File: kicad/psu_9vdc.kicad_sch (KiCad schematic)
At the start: 5 parts, among them U1 LM7809_TO220

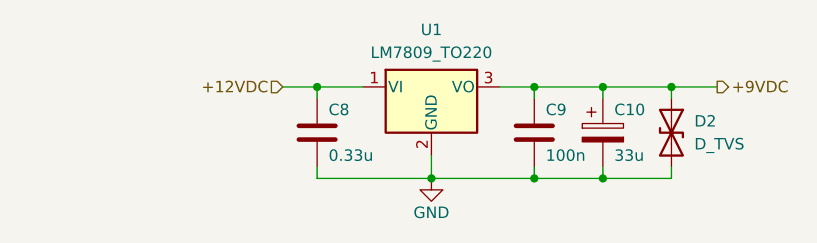
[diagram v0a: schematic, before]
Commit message: Post zip cleanups
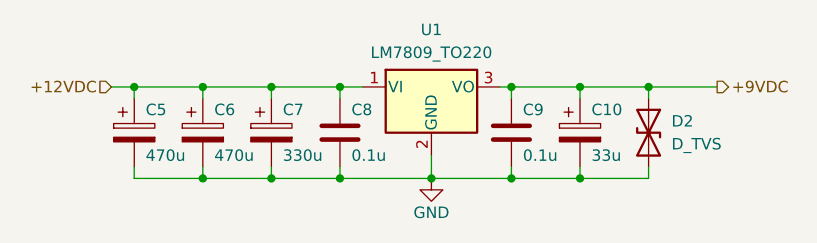
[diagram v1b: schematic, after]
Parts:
- added C5, C6: 470u, cap-470u:ESH_13X20_, symbol Device:C_Polarized
- added C7: 330u, cap-330u:CAPPRD500W60D1000H2200, symbol Device:C_Polarized
- C10: footprint (none) -> cap-33u:EEE0JA152UAP
- C8: value 0.33u -> 0.1u; footprint (none) -> Capacitor_SMD:C_0805_2012Metric
- C9: value 100n -> 0.1u; footprint (none) -> Capacitor_SMD:C_0805_2012Metric
- D2: footprint (none) -> Diode_SMD:D_SOD-523
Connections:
- net +12VDC: now also C5.1, C6.1, C7.1
- net GND: now also C5.2, C6.2, C7.2
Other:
- moved on the sheet: C10, C8, C9, D2
